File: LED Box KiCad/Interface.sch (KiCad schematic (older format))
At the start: 21 parts, among them J301 IR LED, J302 Button, SW301 Reset, SW302 Push 1, SW303 Push 2, U301 ULN2003

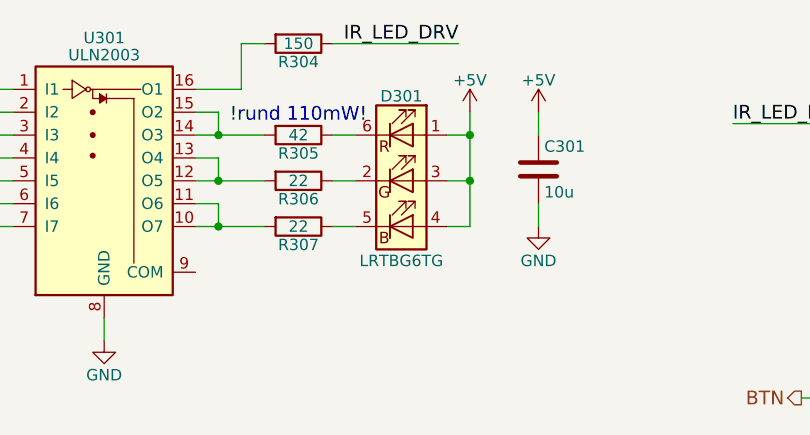
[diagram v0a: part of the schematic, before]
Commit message: Kleine Veränderungen
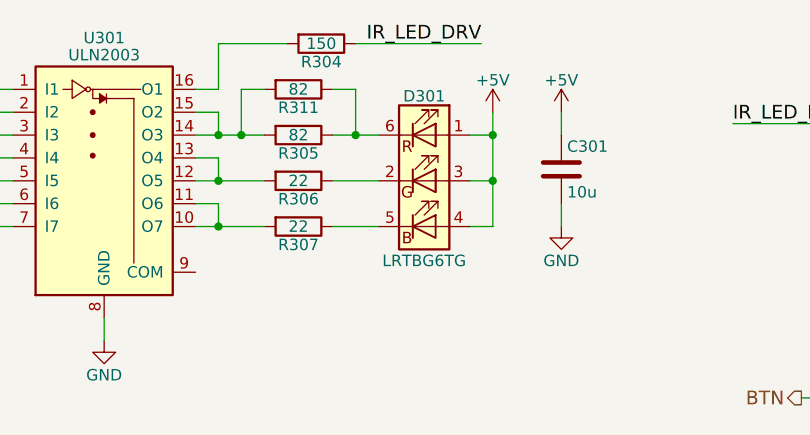
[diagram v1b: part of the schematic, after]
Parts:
- added R311: 82, Resistors_SMD:R_0805, symbol R
- R305: value 42 -> 82
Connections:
- net at R305.2, U301.14 (O3), U301.15 (O2): now also R311.2
- net at D301.6 (RK), R305.1: now also R311.1
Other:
- note removed: "!rund 110mW!"
- moved on the sheet: C301, D301, R304
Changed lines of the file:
@@
 L R R304
 U 1 1 59DBA966
-P 5250 2700
-F 0 "R304" V 5330 2700 50  0000 C CNN
-F 1 "150" V 5250 2700 50  0000 C CNN
-F 2 "Resistors_SMD:R_0805" V 5180 2700 50  0001 C CNN
-F 3 "" H 5250 2700 50  0001 C CNN
-	1    5250 2700
+P 5350 2700
+F 0 "R304" V 5430 2700 50  0000 C CNN
+F 1 "150" V 5350 2700 50  0000 C CNN
+F 2 "Resistors_SMD:R_0805" V 5280 2700 50  0001 C CNN
+F 3 "" H 5350 2700 50  0001 C CNN
+	1    5350 2700
 	0    1    1    0
 $EndComp
@@
 P 5250 3100
 F 0 "R305" V 5330 3100 50  0000 C CNN
-F 1 "42" V 5250 3100 50  0000 C CNN
+F 1 "82" V 5250 3100 50  0000 C CNN
 F 2 "Resistors_SMD:R_0805" V 5180 3100 50  0001 C CNN
 F 3 "" H 5250 3100 50  0001 C CNN
@@
 L +5V #PWR019
 U 1 1 59DBA982
-P 6000 3000
-F 0 "#PWR019" H 6000 2850 50  0001 C CNN
-F 1 "+5V" H 6000 3140 50  0000 C CNN
-F 2 "" H 6000 3000 50  0001 C CNN
-F 3 "" H 6000 3000 50  0001 C CNN
-	1    6000 3000
+P 6100 3000
+F 0 "#PWR019" H 6100 2850 50  0001 C CNN
+F 1 "+5V" H 6100 3140 50  0000 C CNN
+F 2 "" H 6100 3000 50  0001 C CNN
+F 3 "" H 6100 3000 50  0001 C CNN
+	1    6100 3000
 	1    0    0    -1
 $EndComp
@@
 	1    0    0    -1
 $EndComp
-Text Notes 5550 3050 2    60   ~ 0
-!rund 110mW!
 $Comp
 L LRTBG6TG D301
 U 1 1 59DBA991
-P 5700 3300
-F 0 "D301" H 5700 3670 50  0000 C CNN
-F 1 "LRTBG6TG" H 5700 2950 50  0000 C CNN
-F 2 "ledbox-newfootprints:LED-6-BIG" H 5700 2750 50  0001 C CNN
-F 3 "http://www.osram-os.com/Graphics/XPic4/00067263_0.pdf" H 5700 2850 50  0001 C CNN
-	1    5700 3300
-	1    0    0    -1
-$EndComp
-Text Label 5950 2700 2    60   ~ 0
+P 5800 3300
+F 0 "D301" H 5800 3670 50  0000 C CNN
+F 1 "LRTBG6TG" H 5800 2950 50  0000 C CNN
+F 2 "ledbox-newfootprints:LED-6-BIG" H 5800 2750 50  0001 C CNN
+F 3 "http://www.osram-os.com/Graphics/XPic4/00067263_0.pdf" H 5800 2850 50  0001 C CNN
+	1    5800 3300
+	1    0    0    -1
+$EndComp
+Text Label 6050 2700 2    60   ~ 0
 IR_LED_DRV
 Text Label 7150 3050 0    60   ~ 0
@@
 	7450 4250 7850 4250
 Wire Wire Line
-	5950 2700 5400 2700
-Wire Wire Line
-	6000 3100 5900 3100
-Wire Wire Line
-	5400 3500 5500 3500
-Wire Wire Line
-	5400 3300 5500 3300
-Wire Wire Line
-	5400 3100 5500 3100
-Wire Wire Line
-	5000 2700 5100 2700
+	6050 2700 5500 2700
+Wire Wire Line
+	6100 3100 6000 3100
+Wire Wire Line
+	5400 3500 5600 3500
+Wire Wire Line
+	5400 3300 5600 3300
+Wire Wire Line
+	5400 3100 5600 3100
+Wire Wire Line
+	4900 2700 5200 2700
 Wire Wire Line
 	3900 3200 4000 3200
@@
 	4800 3000 4900 3000
 Wire Wire Line
-	4800 2900 5000 2900
-Wire Wire Line
-	5000 2900 5000 2700
+	4800 2900 4900 2900
+Wire Wire Line
+	4900 2900 4900 2700
 Wire Wire Line
 	7150 3050 7850 3050
@@
 Connection ~ 4900 3500
 Wire Wire Line
-	6000 3000 6000 3500
-Wire Wire Line
-	6000 3300 5900 3300
-Connection ~ 6000 3100
-Wire Wire Line
-	6000 3500 5900 3500
-Connection ~ 6000 3300
+	6100 3000 6100 3500
+Wire Wire Line
+	6100 3300 6000 3300
+Connection ~ 6100 3100
+Wire Wire Line
+	6100 3500 6000 3500
+Connection ~ 6100 3300
 $Comp
 L +5V #PWR023
@@
 L +5V #PWR029
 U 1 1 59DBB492
-P 6300 3000
-F 0 "#PWR029" H 6300 2850 50  0001 C CNN
-F 1 "+5V" H 6300 3140 50  0000 C CNN
-F 2 "" H 6300 3000 50  0001 C CNN
-F 3 "" H 6300 3000 50  0001 C CNN
-	1    6300 3000
+P 6400 3000
+F 0 "#PWR029" H 6400 2850 50  0001 C CNN
+F 1 "+5V" H 6400 3140 50  0000 C CNN
+F 2 "" H 6400 3000 50  0001 C CNN
+F 3 "" H 6400 3000 50  0001 C CNN
+	1    6400 3000
 	1    0    0    -1
 $EndComp
@@
 L GND #PWR030
 U 1 1 59DBB498
-P 6300 3500
-F 0 "#PWR030" H 6300 3250 50  0001 C CNN
-F 1 "GND" H 6300 3350 50  0000 C CNN
-F 2 "" H 6300 3500 50  0001 C CNN
-F 3 "" H 6300 3500 50  0001 C CNN
-	1    6300 3500
+P 6400 3500
+F 0 "#PWR030" H 6400 3250 50  0001 C CNN
+F 1 "GND" H 6400 3350 50  0000 C CNN
+F 2 "" H 6400 3500 50  0001 C CNN
+F 3 "" H 6400 3500 50  0001 C CNN
+	1    6400 3500
 	1    0    0    -1
 $EndComp
@@
 L C C301
 U 1 1 59DBB49E
-P 6300 3250
-F 0 "C301" H 6325 3350 50  0000 L CNN
-F 1 "10u" H 6325 3150 50  0000 L CNN
-F 2 "Capacitors_SMD:C_0805" H 6338 3100 50  0001 C CNN
-F 3 "" H 6300 3250 50  0001 C CNN
-	1    6300 3250
-	1    0    0    -1
-$EndComp
-Wire Wire Line
-	6300 3400 6300 3500
-Wire Wire Line
-	6300 3000 6300 3000
-Wire Wire Line
-	6300 3000 6300 3100
+P 6400 3250
+F 0 "C301" H 6425 3350 50  0000 L CNN
+F 1 "10u" H 6425 3150 50  0000 L CNN
+F 2 "Capacitors_SMD:C_0805" H 6438 3100 50  0001 C CNN
+F 3 "" H 6400 3250 50  0001 C CNN
+	1    6400 3250
+	1    0    0    -1
+$EndComp
+Wire Wire Line
+	6400 3400 6400 3500
+Wire Wire Line
+	6400 3000 6400 3000
+Wire Wire Line
+	6400 3000 6400 3100
 $Comp
 L +5V #PWR031
@@
 Wire Wire Line
 	7750 3850 7750 3750
+$Comp
+L R R311
+U 1 1 59E4B05C
+P 5250 2900
+F 0 "R311" V 5330 2900 50  0000 C CNN
+F 1 "82" V 5250 2900 50  0000 C CNN
+F 2 "Resistors_SMD:R_0805" V 5180 2900 50  0001 C CNN
+F 3 "" H 5250 2900 50  0001 C CNN
+	1    5250 2900
+	0    1    1    0
+$EndComp
+Wire Wire Line
+	5100 2900 5000 2900
+Wire Wire Line
+	5000 2900 5000 3100
+Connection ~ 5000 3100
+Wire Wire Line
+	5400 2900 5500 2900
+Wire Wire Line
+	5500 2900 5500 3100
+Connection ~ 5500 3100
 $EndSCHEMATC
